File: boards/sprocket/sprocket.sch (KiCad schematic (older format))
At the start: 1 part, among them U1 STM32G031F8P6

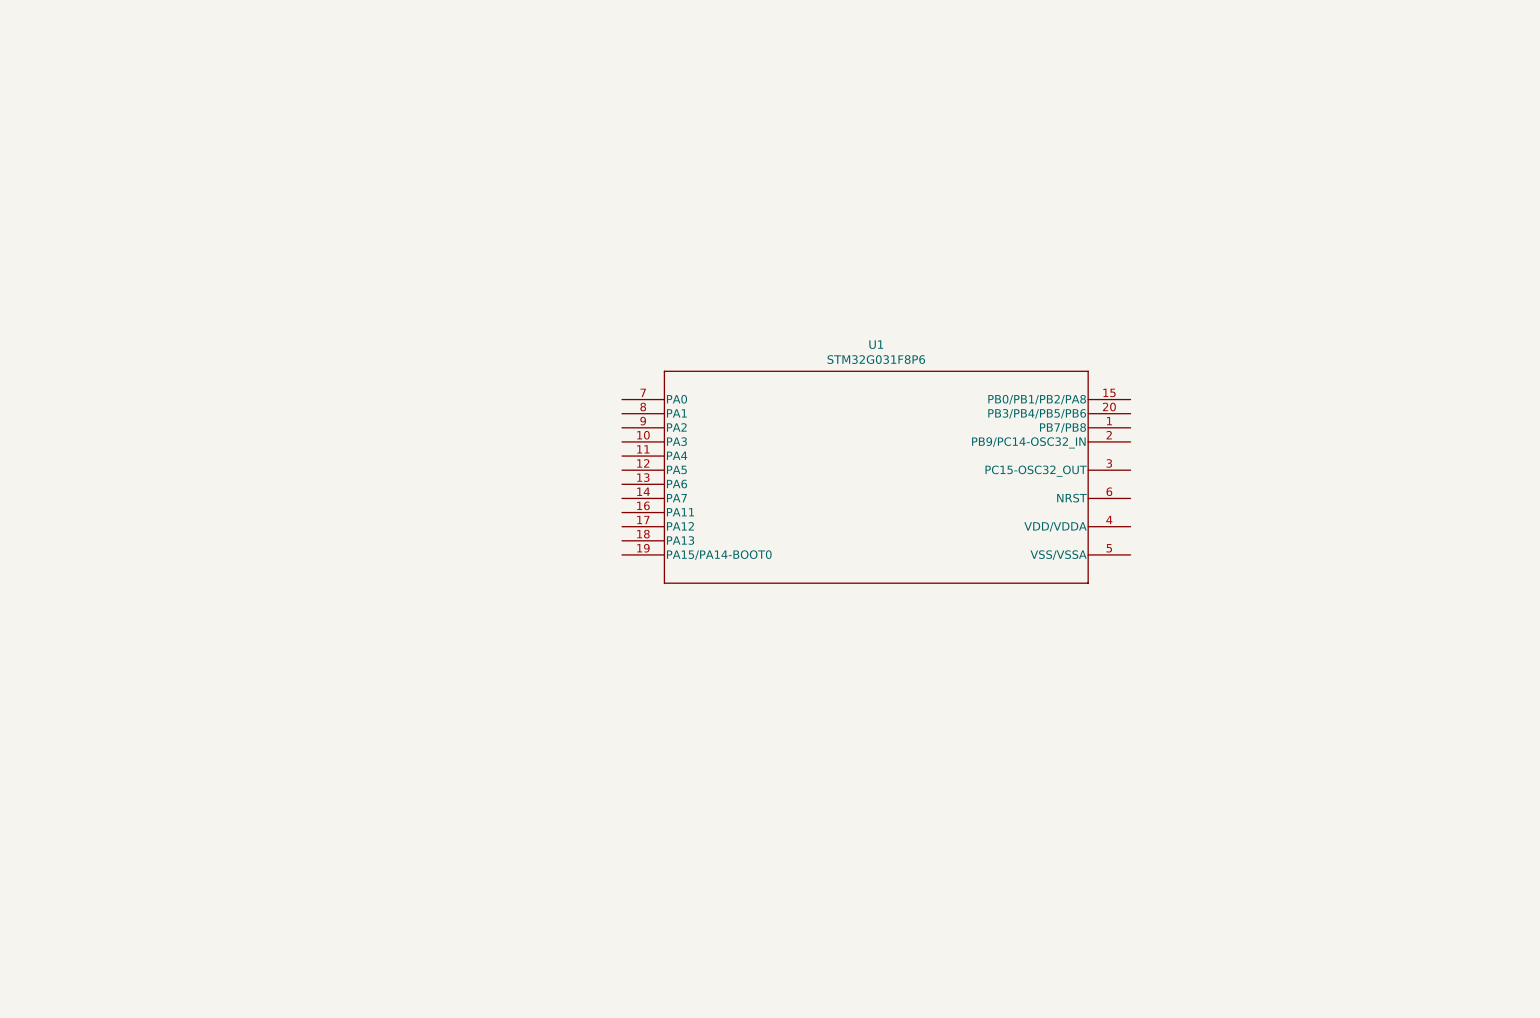
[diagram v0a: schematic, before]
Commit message: Work
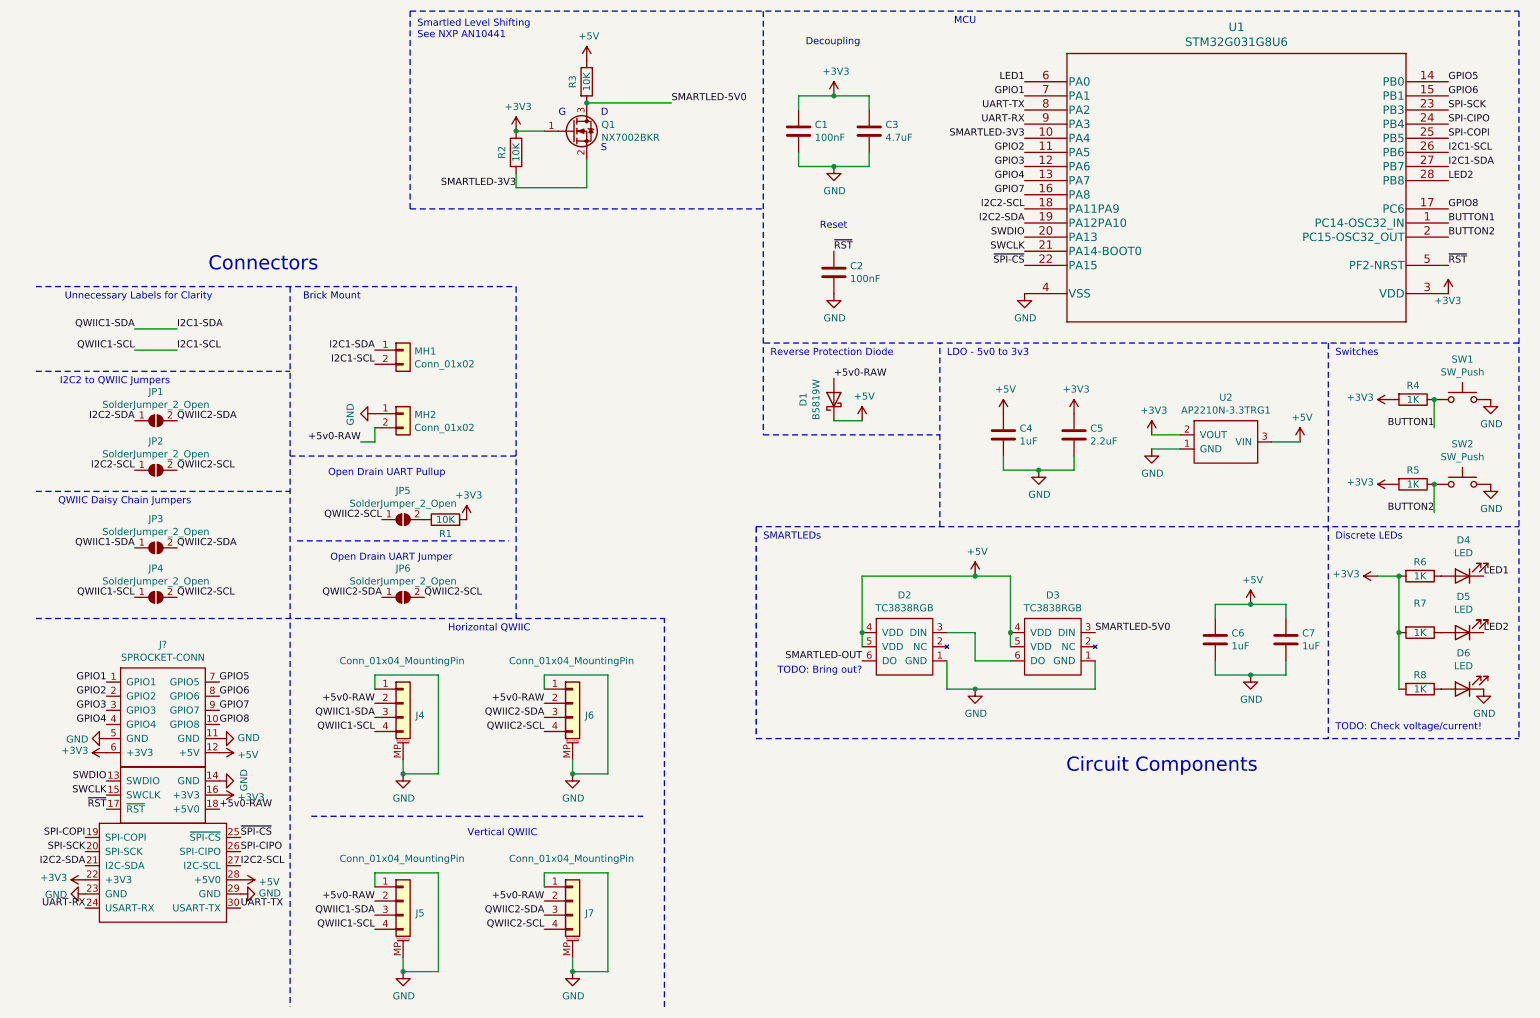
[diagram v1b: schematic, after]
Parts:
- removed U1: STM32G031F8P6, footprints:STM32G031F8P6, symbol stm32g0:STM32G031F8P6
- added C1, C2: 100nF, Capacitor_SMD:C_0402_1005Metric, symbol Device:C
- added C3: 4.7uF, Capacitor_SMD:C_0402_1005Metric, symbol Device:C
- added C4, C6, C7: 1uF, Capacitor_SMD:C_0402_1005Metric, symbol Device:C
- added C5: 2.2uF, Capacitor_SMD:C_0603_1608Metric, symbol Device:C
- added D1: B5819W, Diode_SMD:D_SOD-123, symbol Device:D_Schottky
- added D2, D3: TC3838RGB, Everything:TC3838RGB, symbol Everything:TC3838RGB
- added D4, D5, D6: LED, Diode_SMD:D_0603_1608Metric, symbol Device:LED
- added J4, J6: Conn_01x04_MountingPin, Connector_JST:JST_SH_SM04B-SRSS-TB_1x04-1MP_P1.00mm_Horizontal, symbol Connector_Generic_MountingPin:Conn_01x04_MountingPin
- added J5, J7: Conn_01x04_MountingPin, Connector_JST:JST_SH_BM04B-SRSS-TB_1x04-1MP_P1.00mm_Vertical, symbol Connector_Generic_MountingPin:Conn_01x04_MountingPin
- added J?: SPROCKET-CONN, Everything:sprocket-pins, symbol Everything:SPROCKET-CONN
- added JP1, JP2, JP3, JP4, JP5, JP6: SolderJumper_2_Open, Jumper:SolderJumper-2_P1.3mm_Open_TrianglePad1.0x1.5mm, symbol Jumper:SolderJumper_2_Open
- added MH1, MH2: Conn_01x02, brick-4_9id-6_0od:brick-1x2, symbol Connector_Generic:Conn_01x02
- added Q1: NX7002BKR, Package_TO_SOT_SMD:SOT-23, symbol Device:Q_NMOS_GSD
- added R1, R2, R3: 10K, Resistor_SMD:R_0402_1005Metric, symbol Device:R
- added R4, R5, R6, R7, R8: 1K, Resistor_SMD:R_0402_1005Metric, symbol Device:R
- added SW1, SW2: SW_Push, Everything:K2-1808SN-A4SW-01, symbol Switch:SW_Push
- added U1: STM32G031G8U6, footprints:STM32G031G8U6, symbol STM32G031G8U6:STM32G031G8U6
- added U2: AP2210N-3.3TRG1, Package_TO_SOT_SMD:SOT-23, symbol Everything:AP2210N-3.3TRG1
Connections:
- new net: D2.3 (DIN), D3.6 (DO)
- new net: D4.2 (A), R6.1
- new net: D5.2 (A), R7.1
- new net: D6.2 (A), R8.1
- new net: JP5.2 (B), R1.1
- new net +3V3: C1.1, C3.1, C5.1, J?.16 (+3V3), J?.22 (+3V3), J?.6 (+3V3), Q1.1 (G), R1.2, R2.1, R4.2, R5.2, R6.2, R7.2, R8.2, U1.3 (VDD), U2.2 (VOUT)
- new net +5V: C4.1, C6.1, C7.1, D1.1 (K), D2.4 (VDD), D2.5 (VDD), D3.4 (VDD), D3.5 (VDD), J?.12 (+5V), J?.28 (+5V0), R3.1, U2.3 (VIN)
- new net +5v0-RAW: D1.2 (A), J4.2 (Pin_2), J5.2 (Pin_2), J6.2 (Pin_2), J7.2 (Pin_2), J?.18 (+5V0), MH2.2 (Pin_2)
- new net BUTTON1: R4.1, SW1.1, U1.1 (PC14-OSC32_IN)
- new net BUTTON2: R5.1, SW2.1, U1.2 (PC15-OSC32_OUT)
- new net GND: C1.2, C2.2, C3.2, C4.2, C5.2, C6.2, C7.2, D2.1 (GND), D3.1 (GND), D6.1 (K), J4.1 (Pin_1), J4.MP (MountPin), J5.1 (Pin_1), J5.MP (MountPin), J6.1 (Pin_1), J6.MP (MountPin), J7.1 (Pin_1), J7.MP (MountPin), J?.11 (GND), J?.14 (GND), J?.23 (GND), J?.29 (GND), J?.5 (GND), MH2.1 (Pin_1), SW1.2, SW2.2, U1.4 (VSS), U2.1 (GND)
- new net GPIO1: J?.1 (GPIO1), U1.7 (PA1)
- new net GPIO2: J?.2 (GPIO2), U1.11 (PA5)
- new net GPIO3: J?.3 (GPIO3), U1.12 (PA6)
- new net GPIO4: J?.4 (GPIO4), U1.13 (PA7)
- new net GPIO5: J?.7 (GPIO5), U1.14 (PB0)
- new net GPIO6: J?.8 (GPIO6), U1.15 (PB1)
- new net GPIO7: J?.9 (GPIO7), U1.16 (PA8)
- new net GPIO8: J?.10 (GPIO8), U1.17 (PC6)
- new net I2C1-SCL: J4.4 (Pin_4), J5.4 (Pin_4), JP4.1 (A), MH1.2 (Pin_2), U1.26 (PB6)
- new net I2C1-SDA: J4.3 (Pin_3), J5.3 (Pin_3), JP3.1 (A), MH1.1 (Pin_1), U1.27 (PB7)
- new net I2C2-SCL: J?.27 (I2C-SCL), JP2.1 (A), U1.18 (PA11PA9)
- new net I2C2-SDA: J?.21 (I2C-SDA), JP1.1 (A), U1.19 (PA12PA10)
- new net LED1: D4.1 (K), U1.6 (PA0)
- new net LED2: D5.1 (K), U1.28 (PB8)
- new net QWIIC2-SCL: J6.4 (Pin_4), J7.4 (Pin_4), JP2.2 (B), JP4.2 (B), JP5.1 (A), JP6.2 (B)
- new net QWIIC2-SDA: J6.3 (Pin_3), J7.3 (Pin_3), JP1.2 (B), JP3.2 (B), JP6.1 (A)
- new net SMARTLED-3V3: Q1.2 (S), R2.2, U1.10 (PA4)
- new net SMARTLED-5V0: D3.3 (DIN), Q1.3 (D), R3.2
- new net SMARTLED-OUT: D2.6 (DO)
- new net SPI-CIPO: J?.26 (SPI-CIPO), U1.24 (PB4)
- new net SPI-COPI: J?.19 (SPI-COPI), U1.25 (PB5)
- new net SPI-SCK: J?.20 (SPI-SCK), U1.23 (PB3)
- new net SWCLK: J?.15 (SWCLK), U1.21 (PA14-BOOT0)
- new net SWDIO: J?.13 (SWDIO), U1.20 (PA13)
- new net UART-RX: J?.24 (USART-RX), U1.9 (PA3)
- new net UART-TX: J?.30 (USART-TX), U1.8 (PA2)
- new net ~RST: C2.1, J?.17 (~RST), U1.5 (PF2-NRST)
- new net ~SPI-CS: J?.25 (~SPI-CS), U1.22 (PA15)
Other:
- note added: "Brick Mount"
- note added: "Circuit Components"
- note added: "Connectors"
- note added: "D"
- note added: "Decoupling"
- note added: "Discrete LEDs"
- note added: "G"
- note added: "Horizontal QWIIC"
- note added: "I2C2 to QWIIC Jumpers"
- note added: "LDO - 5v0 to 3v3"
- note added: "MCU"
- note added: "Open Drain UART Jumper"
- note added: "Open Drain UART Pullup\n"
- note added: "QWIIC Daisy Chain Jumpers"
- note added: "Reset"
- note added: "Reverse Protection Diode"
- note added: "S"
- note added: "SMARTLEDs"
- note added: "Smartled Level Shifting\nSee NXP AN10441"
- note added: "Switches"
- note added: "TODO: Bring out?"
- note added: "TODO: Check voltage/current!"
- note added: "Unnecessary Labels for Clarity"
- note added: "Vertical QWIIC"

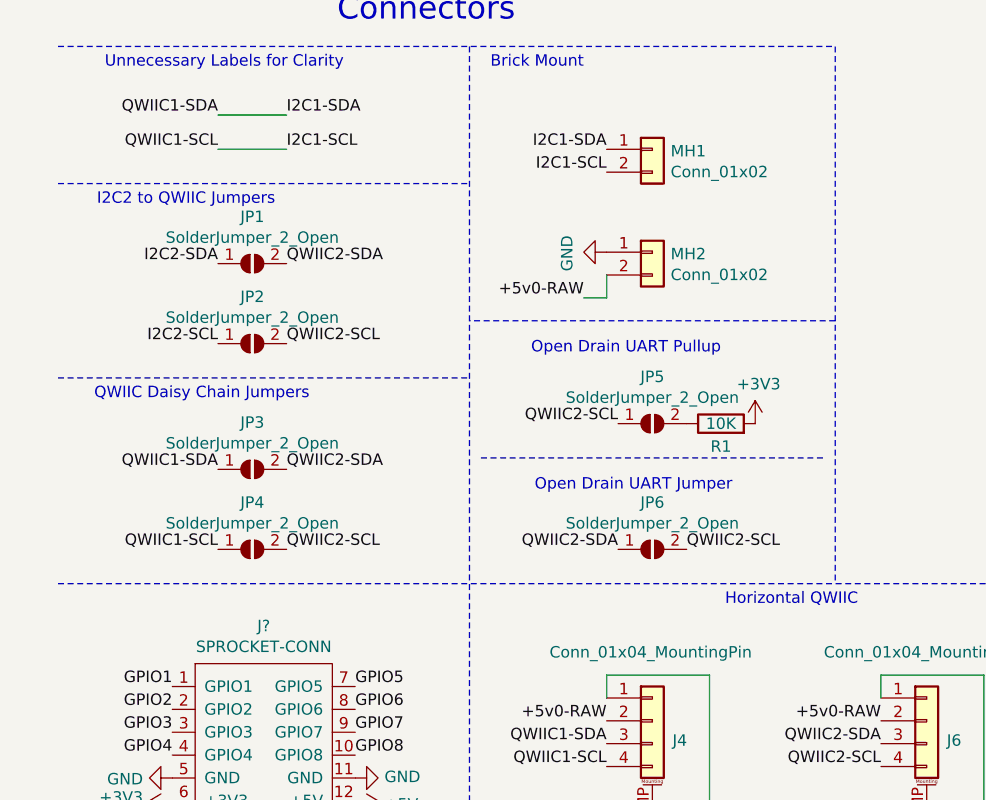
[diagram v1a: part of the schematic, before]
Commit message: About to give up again
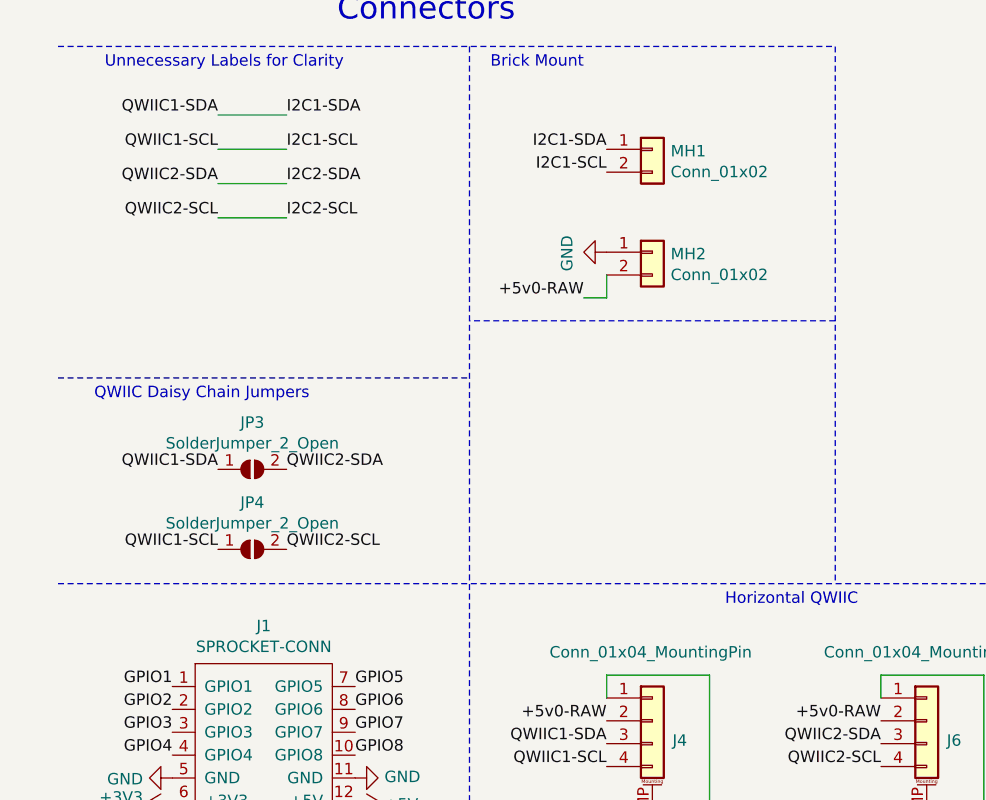
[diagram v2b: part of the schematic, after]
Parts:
- removed JP1, JP2, JP5, JP6: SolderJumper_2_Open, Jumper:SolderJumper-2_P1.3mm_Open_TrianglePad1.0x1.5mm, symbol Jumper:SolderJumper_2_Open
- removed R1: 10K, Resistor_SMD:R_0402_1005Metric, symbol Device:R
- gave numbers to parts that had none: 1
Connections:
- net QWIIC2-SCL is gone; now on net I2C2-SCL: J6.4 (Pin_4), J7.4 (Pin_4), JP4.2 (B)
- net QWIIC2-SDA is gone; now on net I2C2-SDA: J6.3 (Pin_3), J7.3 (Pin_3), JP3.2 (B)
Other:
- note removed: "I2C2 to QWIIC Jumpers"
- note removed: "Open Drain UART Jumper"
- note removed: "Open Drain UART Pullup\n"
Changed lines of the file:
@@
 Text Notes 1600 4200 2    50   ~ 0
 QWIIC Daisy Chain Jumpers
-$Comp
-L Jumper:SolderJumper_2_Open JP6
-U 1 1 6067FFF6
-P 3100 4850
-F 0 "JP6" H 3100 5055 50  0000 C CNN
-F 1 "SolderJumper_2_Open" H 3100 4964 50  0000 C CNN
-F 2 "Jumper:SolderJumper-2_P1.3mm_Open_TrianglePad1.0x1.5mm" H 3100 4850 50  0001 C CNN
-F 3 "~" H 3100 4850 50  0001 C CNN
-	1    3100 4850
-	1    0    0    -1
-$EndComp
-Text Label 2950 4850 2    50   ~ 0
-QWIIC2-SDA
-Text Label 3250 4850 0    50   ~ 0
-QWIIC2-SCL
-Text Notes 3450 4600 2    50   ~ 0
-Open Drain UART Jumper
-$Comp
-L Jumper:SolderJumper_2_Open JP5
-U 1 1 6069AF59
-P 3100 4300
-F 0 "JP5" H 3100 4505 50  0000 C CNN
-F 1 "SolderJumper_2_Open" H 3100 4414 50  0000 C CNN
-F 2 "Jumper:SolderJumper-2_P1.3mm_Open_TrianglePad1.0x1.5mm" H 3100 4300 50  0001 C CNN
-F 3 "~" H 3100 4300 50  0001 C CNN
-	1    3100 4300
-	1    0    0    -1
-$EndComp
-$Comp
-L Device:R R1
-U 1 1 606A0041
-P 3400 4300
-F 0 "R1" V 3300 4300 50  0000 C CNN
-F 1 "10K" V 3400 4300 50  0000 C CNN
-F 2 "Resistor_SMD:R_0402_1005Metric" V 3330 4300 50  0001 C CNN
-F 3 "~" H 3400 4300 50  0001 C CNN
-	1    3400 4300
-	0    -1   -1   0
-$EndComp
-$Comp
-L power:+3V3 #PWR0135
-U 1 1 606A1D31
-P 3550 4300
-F 0 "#PWR0135" H 3550 4150 50  0001 C CNN
-F 1 "+3V3" H 3565 4473 50  0000 C CNN
-F 2 "" H 3550 4300 50  0001 C CNN
-F 3 "" H 3550 4300 50  0001 C CNN
-	1    3550 4300
-	1    0    0    -1
-$EndComp
-Text Label 2950 4300 2    50   ~ 0
-QWIIC2-SCL
-Text Notes 3400 4000 2    50   ~ 0
-Open Drain UART Pullup\n
 Wire Notes Line
 	3900 3850 2300 3850
@@
 Text Label 1500 2950 0    50   ~ 0
 I2C1-SDA
-$Comp
-L Jumper:SolderJumper_2_Open JP1
-U 1 1 606C75BE
-P 1350 3600
-F 0 "JP1" H 1350 3805 50  0000 C CNN
-F 1 "SolderJumper_2_Open" H 1350 3714 50  0000 C CNN
-F 2 "Jumper:SolderJumper-2_P1.3mm_Open_TrianglePad1.0x1.5mm" H 1350 3600 50  0001 C CNN
-F 3 "~" H 1350 3600 50  0001 C CNN
-	1    1350 3600
-	1    0    0    -1
-$EndComp
-$Comp
-L Jumper:SolderJumper_2_Open JP2
-U 1 1 606C75C4
-P 1350 3950
-F 0 "JP2" H 1350 4155 50  0000 C CNN
-F 1 "SolderJumper_2_Open" H 1350 4064 50  0000 C CNN
-F 2 "Jumper:SolderJumper-2_P1.3mm_Open_TrianglePad1.0x1.5mm" H 1350 3950 50  0001 C CNN
-F 3 "~" H 1350 3950 50  0001 C CNN
-	1    1350 3950
-	1    0    0    -1
-$EndComp
-Text Label 1500 3600 0    50   ~ 0
+Text Label 1200 3250 2    50   ~ 0
 QWIIC2-SDA
-Text Label 1500 3950 0    50   ~ 0
+Text Label 1200 3400 2    50   ~ 0
 QWIIC2-SCL
-Text Label 1200 3600 2    50   ~ 0
+Text Label 1500 3250 0    50   ~ 0
 I2C2-SDA
-Text Label 1200 3950 2    50   ~ 0
+Text Label 1500 3400 0    50   ~ 0
 I2C2-SCL
 Wire Wire Line
@@
 	1200 3100 1500 3100
 Wire Notes Line
-	500  3250 2300 3250
-Wire Notes Line
 	2300 2650 2300 7750
-Text Notes 1450 3350 2    50   ~ 0
-I2C2 to QWIIC Jumpers
 Text Notes 1750 2750 2    50   ~ 0
 Unnecessary Labels for Clarity
@@
 Text Label 1950 7050 0    50   ~ 0
 UART-TX
-Wire Notes Line
-	2350 4450 3850 4450
 $Comp
 L Connector_Generic:Conn_01x02 MH1
@@
 Circuit Components
 $Comp
-L Everything:SPROCKET-CONN J?
+L Everything:SPROCKET-CONN J1
 U 1 1 607795BD
 P 1400 5350
-F 0 "J?" H 1400 5515 50  0000 C CNN
+F 0 "J1" H 1400 5515 50  0000 C CNN
 F 1 "SPROCKET-CONN" H 1400 5424 50  0000 C CNN
 F 2 "Everything:sprocket-pins" H 1400 5400 50  0001 C CNN
@@
 	1    0    0    -1
 $EndComp
+Wire Wire Line
+	1500 3250 1200 3250
+Wire Wire Line
+	1500 3400 1200 3400
 $EndSCHEMATC
